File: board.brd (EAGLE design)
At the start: 88.6 x 95.2 mm, 36 parts, among them K1 RT444012, K2 RT444012, K3 G5LE, Q1 200mA/40V, Q2 200mA/40V, Q3 200mA/40V

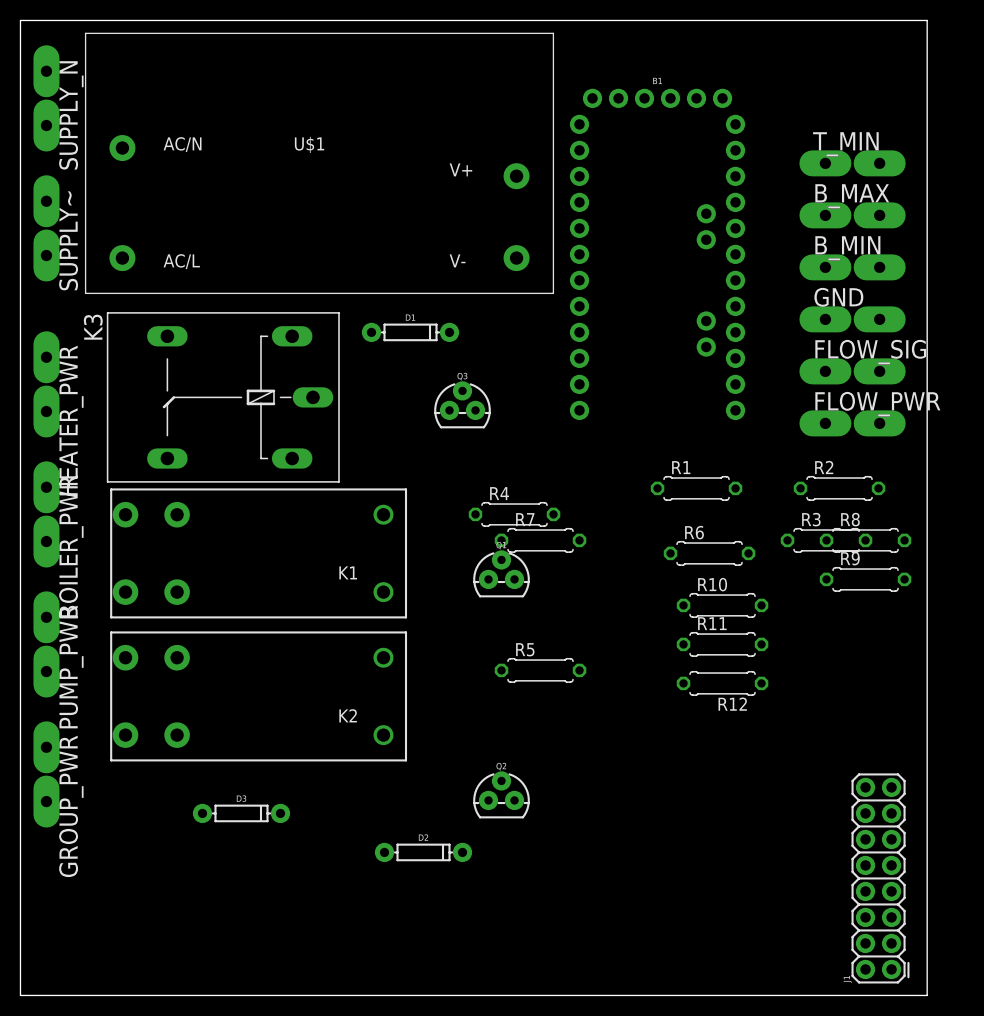
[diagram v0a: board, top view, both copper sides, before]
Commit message: did routing. fixed floating buttons. added drill guide?
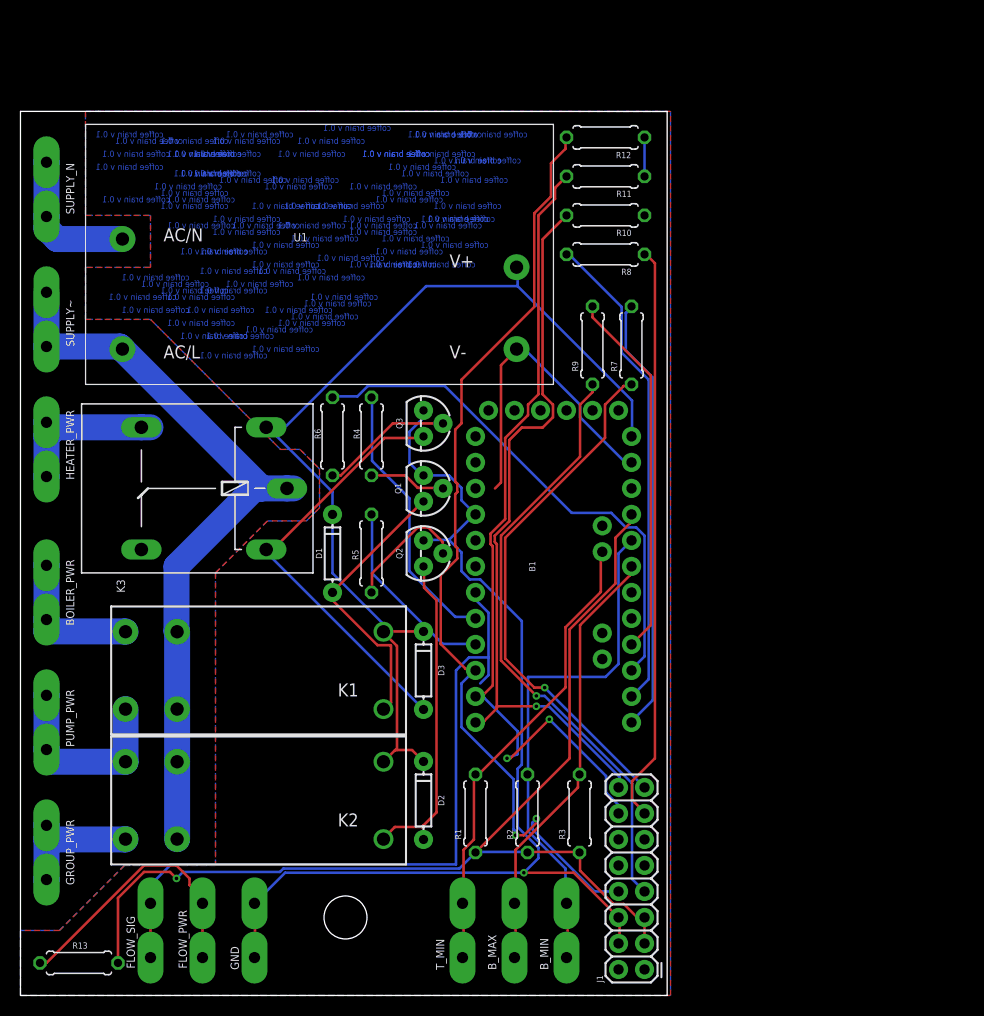
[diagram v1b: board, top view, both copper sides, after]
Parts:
- removed U$1: (no value), meanwell_irm_v5:IRM_05/10
- added R13: (no value), rcl:0207/7
- added U1: 12VDC, meanwell_irm_v5:IRM_05/10
- moved FLOW_SIG 87.7 mm to (12.7, 6.35), turned to 90 degrees
- moved T_MIN 84.1 mm to (43.2, 6.35), turned to 90 degrees
- moved GND 83.5 mm to (22.9, 6.35), turned to 90 degrees
- moved FLOW_PWR 80.5 mm to (17.8, 6.35), turned to 90 degrees
- moved B_MAX 77.3 mm to (48.3, 6.35), turned to 90 degrees
- moved B_MIN 70.5 mm to (53.3, 6.35), turned to 90 degrees
- moved R12 54.6 mm to (57.1, 83.8), turned to 0 degrees
- moved R11 47.1 mm to (57.1, 80.0), turned to 180 degrees
- moved R2 44.0 mm to (49.5, 17.8), turned to 90 degrees
- moved R10 39.8 mm to (57.1, 76.2), turned to 180 degrees
- moved R6 38.6 mm to (30.5, 54.6), turned to 90 degrees
- moved R1 38.4 mm to (44.5, 17.8), turned to 90 degrees
- moved R8 37.8 mm to (57.1, 72.4), turned to 180 degrees
- moved R3 36.0 mm to (54.6, 17.8), turned to 90 degrees
- moved R9 35.1 mm to (55.9, 63.5), turned to 90 degrees
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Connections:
- net N$8 renamed FLOW_SIG
- removed net N$1: J1.16, R10.1
- removed net N$22: J1.14, R11.2
- removed net N$4: J1.8, R12.1
- new net SUPPLY_N: SUPPLY_N.A1, SUPPLY_N.A2, U1.AC/N
- net DBL_BTN: now also J1.14, R11.2; no longer R11.1
- net DBL_LED: now also R8.2; no longer R8.1
- net GND: now also R10.1, R11.1, R12.2, U1.V-; no longer U$1.V-
- net N$14: now also R9.1; no longer R9.2
- net N$23: now also R8.1; no longer R8.2
- net N$24: now also R7.1; no longer R7.2
- net N$3: now also FLOW_PWR.A1, FLOW_PWR.A2, R13.1; no longer SUPPLY_N.A1, SUPPLY_N.A2, U$1.AC/N
- net RAW: now also U1.V+; no longer U$1.V+
- net SNGL_BTN: now also J1.16
- net SNGL_LED: now also R7.2; no longer R7.1
- net STOP_BTN: now also J1.8, R12.1; no longer R12.2
- net STOP_LED: now also R9.2; no longer R9.1
- net SUPPLY: now also U1.AC/L; no longer U$1.AC/L
- net T_MIN: now also R1.2; no longer R1.1
- net VCC: now also R1.1, R13.2; no longer FLOW_PWR.A1, FLOW_PWR.A2, R1.2
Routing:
- net GND: track 0.00 -> 141.9 mm, vias 0 -> 1
- net VCC: track 0.00 -> 105.8 mm, vias 0 -> 1
- net RAW: track 0.00 -> 98.1 mm
- net STOP_BTN: track 0.00 -> 93.4 mm, vias 0 -> 2
- net DBL_BTN: track 0.00 -> 81.6 mm, vias 0 -> 2
- net SUPPLY: track 0.00 -> 74.5 mm
- net SNGL_BTN: track 0.00 -> 71.8 mm, vias 0 -> 1
- net FLOW_SIG: track 0.00 -> 70.2 mm
- net N$14: track 0.00 -> 59.5 mm, vias 0 -> 1
- net N$23: track 0.00 -> 56.8 mm
- net N$24: track 0.00 -> 51.1 mm, vias 0 -> 1
- net B_MIN: track 0.00 -> 51.0 mm
- net HEAT: track 0.00 -> 50.7 mm
- net DBL_LED: track 0.00 -> 47.5 mm
- net T_MIN: track 0.00 -> 45.7 mm
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- added copper zone on layer 1, net GND
- added copper zone on layer 16, net GND
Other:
- board size 88.6 x 95.2 mm -> 63.2 x 86.4 mm
- board text added: "by stewart jackson"
- board text added: "coffee brain v 0.1"
